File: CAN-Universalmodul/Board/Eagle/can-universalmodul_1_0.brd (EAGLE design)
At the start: 100 x 50 mm, 51 parts, among them IC1 MCP 2562, IC2 MCP 2515, IC3 ATMEGA 328P, Q1 16M, Q2 16M, X1 MINI-USB-UX60-MB-5ST, X4 B4B-ZR

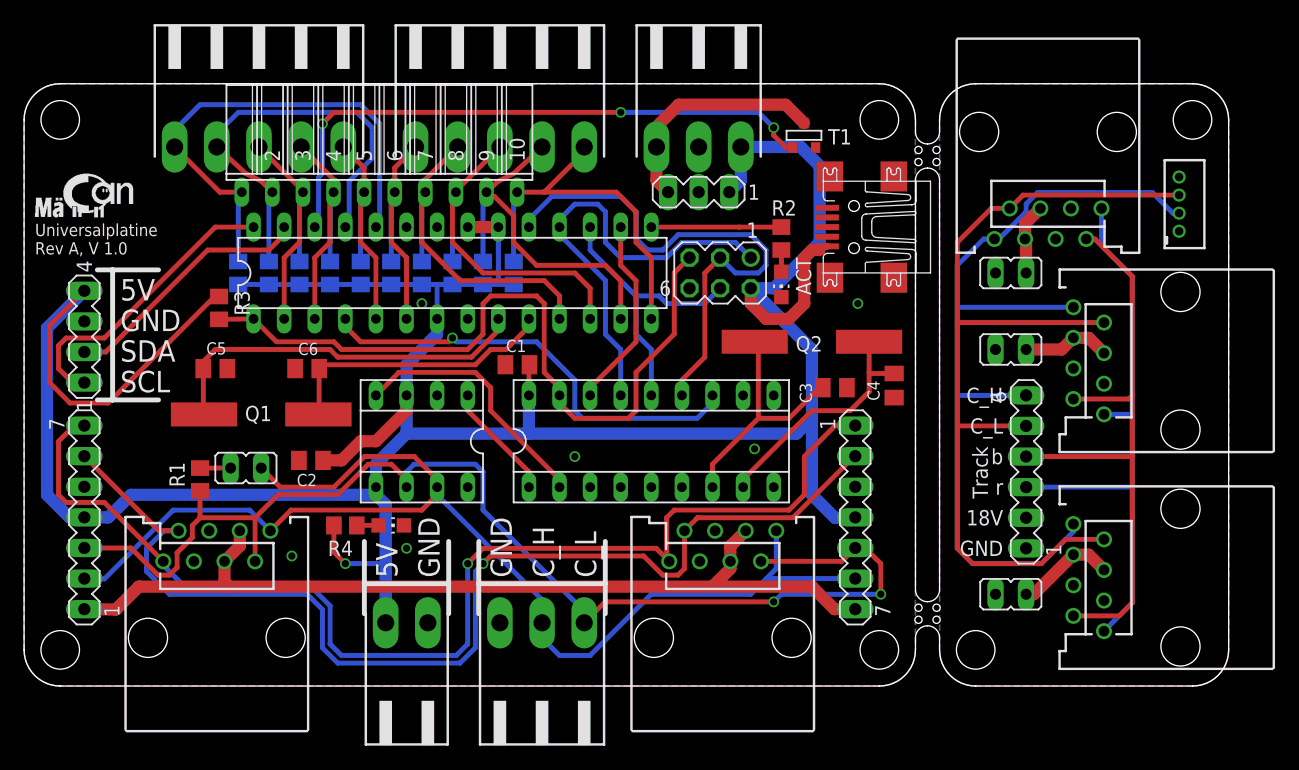
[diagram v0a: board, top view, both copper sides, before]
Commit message: Anpassungen
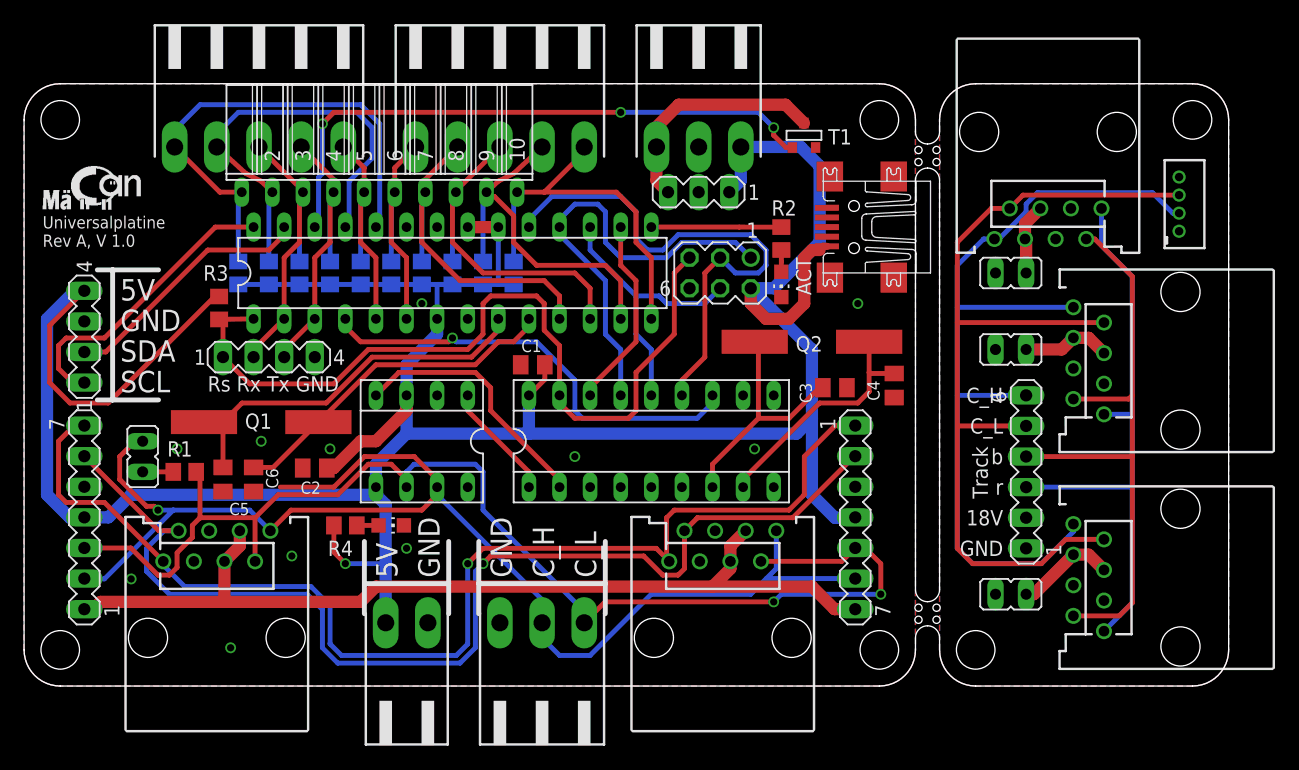
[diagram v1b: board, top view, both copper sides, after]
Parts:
- added SV3: Serial, con-lstb:MA04-1
- moved C6 10.2 mm to (19.1, 17.1), turned to 90 degrees
- moved C5 9.23 mm to (16.5, 17.1), turned to 90 degrees
- moved JP1 8.63 mm to (9.84, 19.1), turned to 0 degrees
- moved R1 1.42 mm to (13.3, 17.8), turned to 180 degrees
- moved C1 1.27 mm to (42.2, 26.7)
- moved C2 0.71 mm to (24.1, 18.1)
- moved Q1 0.64 mm to (19.7, 21.9)
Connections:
- net 7: now also SV3.3
- net 8: now also SV3.2
- net GND: now also SV3.4
- net RESET: now also SV3.1
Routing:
- net CAN-H: track 101.7 -> 109.2 mm, vias 0 -> 1
- net RESET: track 62.1 -> 68.9 mm
- net N$8: track 23.9 -> 28.5 mm
- net 8: track 22.3 -> 26.5 mm
- net 7: track 21.9 -> 26.1 mm
- net CAN-L: track 103.0 -> 105.0 mm
- net 18V: track 76.7 -> 77.8 mm
- net VCC: track 255.2 -> 256.1 mm
- net N$7: track 32.0 -> 32.7 mm
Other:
- board text added: "Rs Rx Tx GND"

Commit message: PCB-Production-Ready
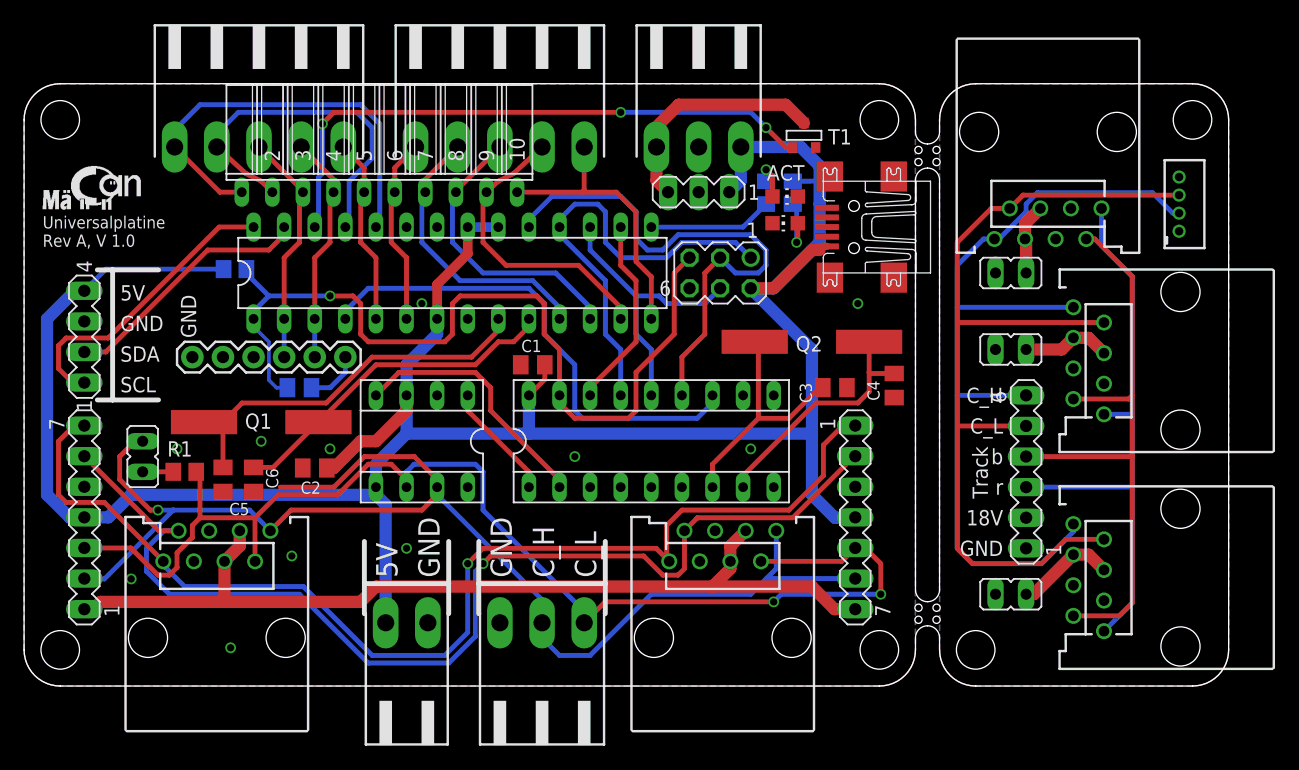
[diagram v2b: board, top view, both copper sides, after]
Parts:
- removed R10, R11, R12, R13, R14, R5, R6, R7, R8, R9: 10k, rcl:R0805
- removed SV3: Serial, con-lstb:MA04-1
- added C7: 100n, rcl:C0805K
- added J6: FTDI_BASICPTH, SparkFun-Connectors:FTDI_BASIC
- moved R4 46.3 mm to (63.8, 41.0), flipped to the bottom, turned to 90 degrees
- moved PWR 41.2 mm to (63.2, 38.4), turned to 90 degrees
- moved ACT 7.31 mm to (63.2, 40.6), turned to 270 degrees
- moved R2 4.02 mm to (61.6, 41.0), flipped to the bottom, turned to 270 degrees
- moved R3 3.48 mm to (17.5, 34.6), flipped to the bottom, turned to 0 degrees
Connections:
- new net N$17: C7.2, J6.DTR
- net 1: no longer R5.1
- net 10: no longer R14.1
- net 2: no longer R6.1
- net 3: no longer R7.1
- net 4: no longer R8.1
- net 5: no longer R9.1
- net 6: no longer R10.1
- net 7: now also J6.RXI; no longer R11.1, SV3.3
- net 8: now also J6.TXO; no longer R12.1, SV3.2
- net 9: no longer R13.1
- net GND: now also J6.GND; no longer SV3.4
- net RESET: now also C7.1; no longer SV3.1
- net VCC: no longer R10.2, R11.2, R12.2, R13.2, R14.2, R5.2, R6.2, R7.2, R8.2, R9.2
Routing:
- net VCC: track 256.1 -> 209.7 mm, vias 1 -> 0
- net 3: track 31.0 -> 24.2 mm
- net 1: track 31.0 -> 24.2 mm
- net 8: track 26.5 -> 20.0 mm
- net 7: track 26.1 -> 19.6 mm
- net 4: track 30.2 -> 23.8 mm
- net 9: track 36.4 -> 30.9 mm
- net 10: track 41.7 -> 36.2 mm
- net 6: track 21.5 -> 16.0 mm
- net 5: track 21.5 -> 16.0 mm
- net 2: track 30.5 -> 25.3 mm
- net N$17: track 0.00 -> 4.61 mm
- net INT: track 37.2 -> 41.3 mm, vias 1 -> 0
- net RESET: track 68.9 -> 72.5 mm, vias 0 -> 1
- net RT: track 97.8 -> 94.7 mm
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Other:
- board text removed: "Rs Rx Tx GND"
